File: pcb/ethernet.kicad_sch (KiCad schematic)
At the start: 1 part, among them U57 ENC28J60x-SP

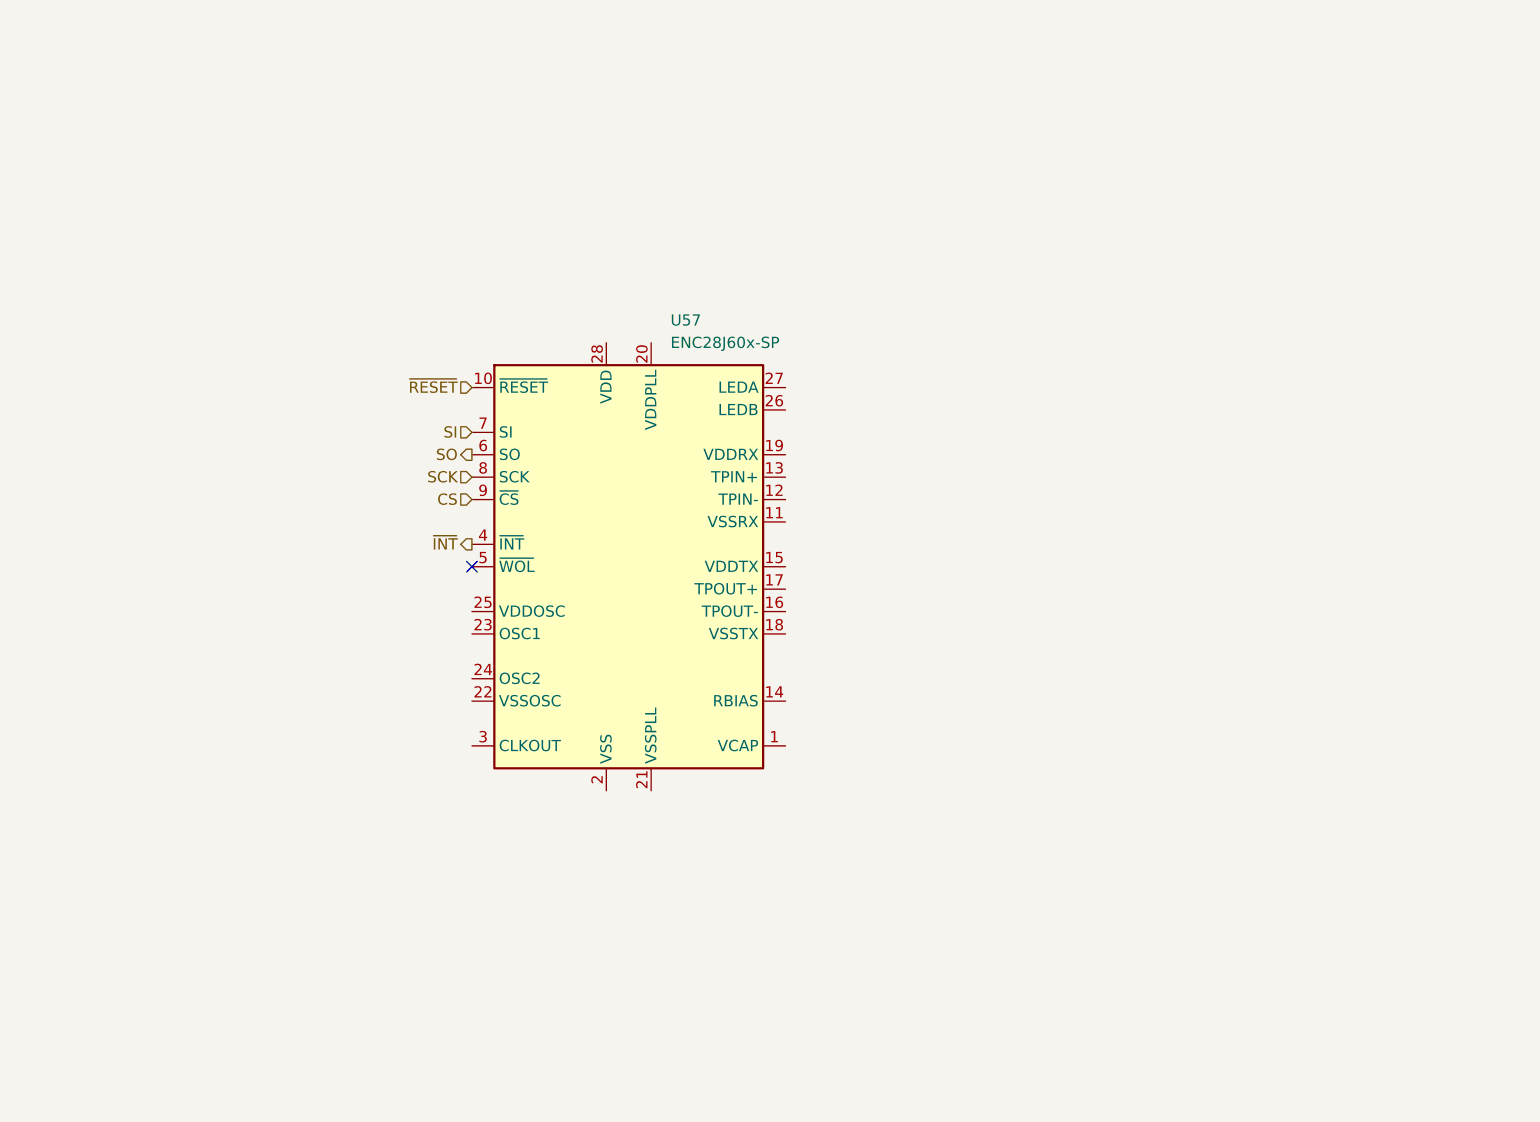
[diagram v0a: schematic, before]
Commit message: WIP schematic
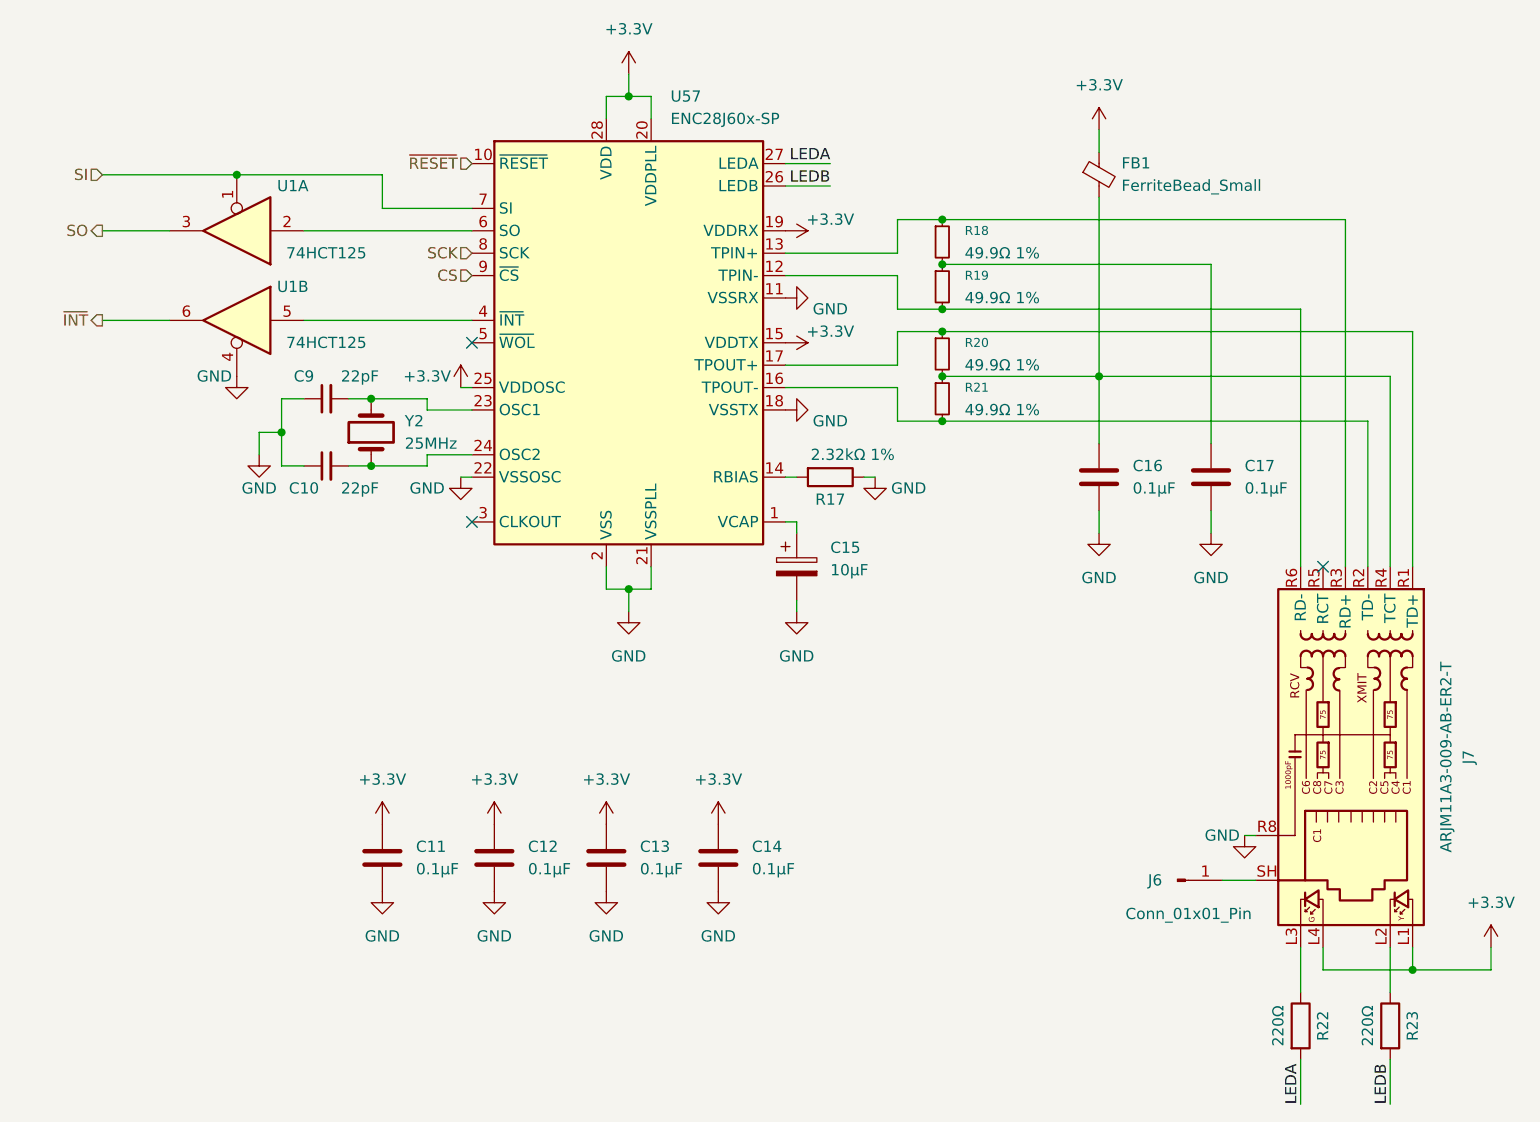
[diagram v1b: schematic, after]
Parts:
- added C10, C9: 22pF, symbol Device:C_Small
- added C11, C12, C13, C14, C16, C17: 0.1µF, symbol Device:C
- added C15: 10µF, symbol Device:C_Polarized
- added FB1: FerriteBead_Small, symbol Device:FerriteBead_Small
- added J6: Conn_01x01_Pin, symbol Connector:Conn_01x01_Pin
- added J7: ARJM11A3-009-AB-ER2-T, Connector_RJ:RJ45_Amphenol_RJMG1BD3B8K1ANR, symbol Connector:RJ45_Amphenol_RJMG1BD3B8K1ANR
- added R17: 2.32kΩ 1%, symbol Device:R
- added R18, R19, R20, R21: 49.9Ω 1%, symbol Device:R_Small
- added R22, R23: 220Ω, symbol Device:R
- added U1: 74HCT125, symbol 74xx:74LS125
- added Y2: 25MHz, symbol Device:Crystal
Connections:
- net SI: now also U1.1
- net SO: now also U1.3; no longer U57.6 (SO)
- net ~{INT}: now also U1.6; no longer U57.4 (~{INT})
- net at U57.1 (VCAP): now also C15.1
- net GND: now reaches U57.11 (VSSRX)
- net GND: now also U57.18 (VSSTX), U57.2 (VSS), U57.21 (VSSPLL), U57.22 (VSSOSC), C10.1, C11.2, C12.2, C13.2, C14.2, C15.2, C16.2, C17.2, C9.1, J7.R8, R17.1, U1.4
- net at U57.12 (TPIN-): now also J7.R6 (RD-), R19.2
- net at U57.13 (TPIN+): now also J7.R3 (RD+), R18.1
- net at U57.14 (RBIAS): now also R17.2
- net +3.3V: now reaches U57.15 (VDDTX)
- net +3.3V: now also U57.19 (VDDRX), U57.20 (VDDPLL), U57.25 (VDDOSC), U57.28 (VDD), C11.1, C12.1, C13.1, C14.1, FB1.1, J7.L1, J7.L4
- net at U57.16 (TPOUT-): now also J7.R2 (TD-), R21.2
- net at U57.17 (TPOUT+): now also J7.R1 (TD+), R20.1
- net at U57.23 (OSC1): now also C9.2, Y2.2
- net at U57.24 (OSC2): now also C10.2, Y2.1
- net LEDB: now reaches U57.26 (LEDB)
- net LEDB: now also R23.2
- net LEDA: now reaches U57.27 (LEDA)
- net LEDA: now also R22.2
- new net: C16.1, FB1.2, J7.R4 (TCT), R20.2, R21.1
- new net: U1.5, U57.4 (~{INT})
- new net: C17.1, R18.2, R19.1
- new net: J6.1 (Pin_1), J7.SH
- new net: J7.L3, R22.1
- new net: J7.L2, R23.1
- new net: U1.2, U57.6 (SO)
- no-connect marks 1 -> 3
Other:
- moved on the sheet: U57
